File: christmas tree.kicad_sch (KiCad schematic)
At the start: 9 parts, among them SW1 SW_SPST

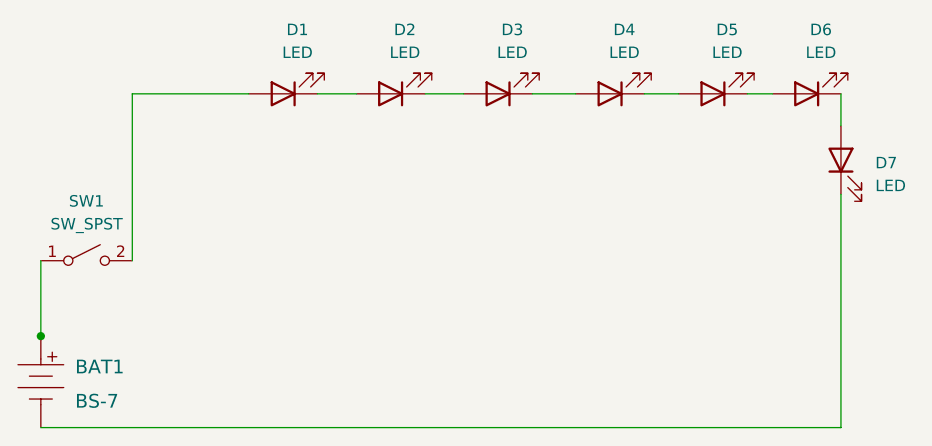
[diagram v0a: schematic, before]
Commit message: retraced the circuit
still don't know if this will work
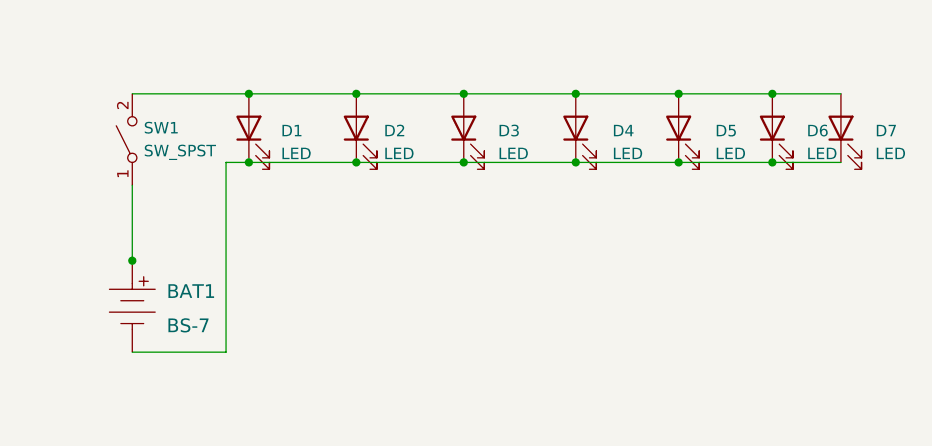
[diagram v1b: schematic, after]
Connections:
- net at D2.1 (K): now also BAT1.Neg, D1.1 (K), D3.1 (K), D4.1 (K), D5.1 (K), D6.1 (K), D7.1 (K); no longer D3.2 (A)
- net at D2.2 (A): now also D1.2 (A), D3.2 (A), D4.2 (A), D5.2 (A), D6.2 (A), D7.2 (A), SW1.2 (B); no longer D1.1 (K)
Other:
- moved on the sheet: BAT1, D1, D2, D3, D4, D5, D6, D7, SW1
